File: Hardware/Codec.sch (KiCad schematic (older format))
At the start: 11 parts, among them U301 SGTL5000XNAA3

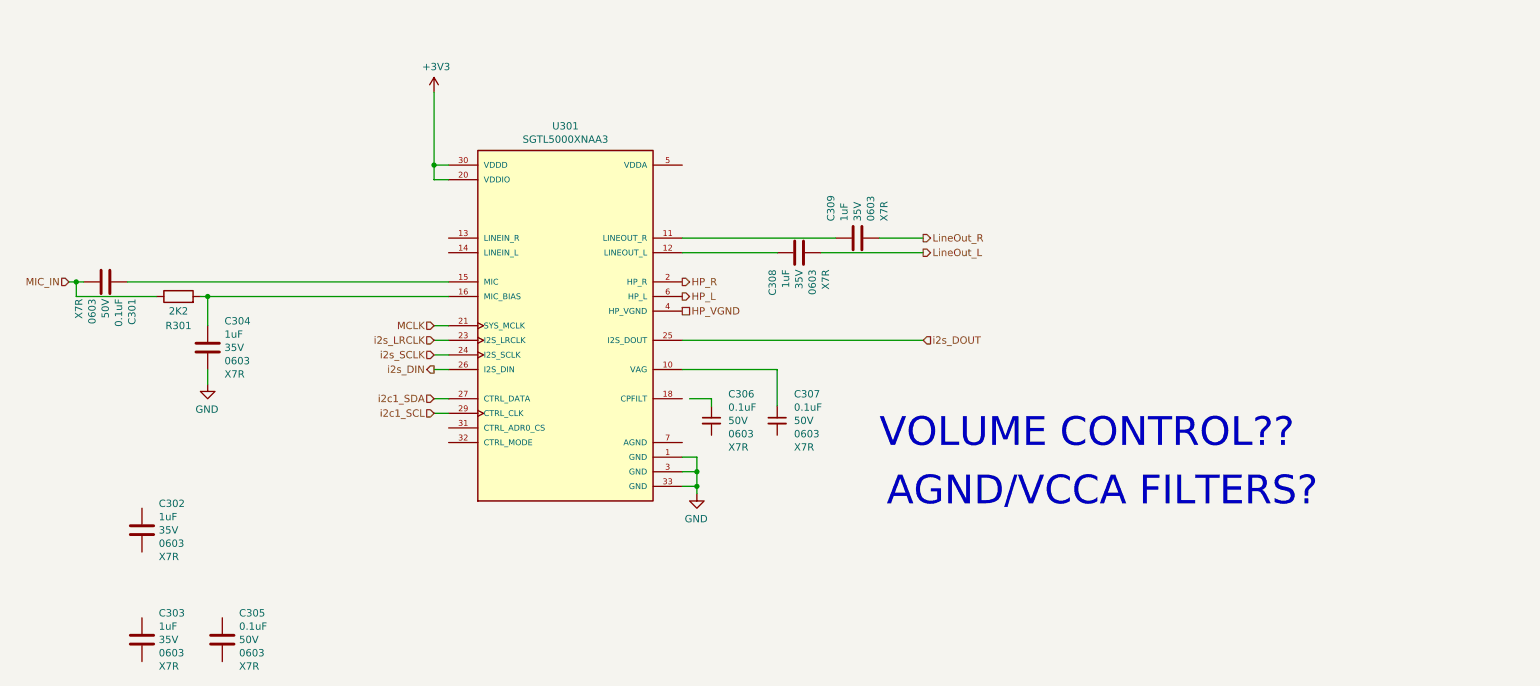
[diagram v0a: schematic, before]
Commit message: Commit berfore merge back with power fix.
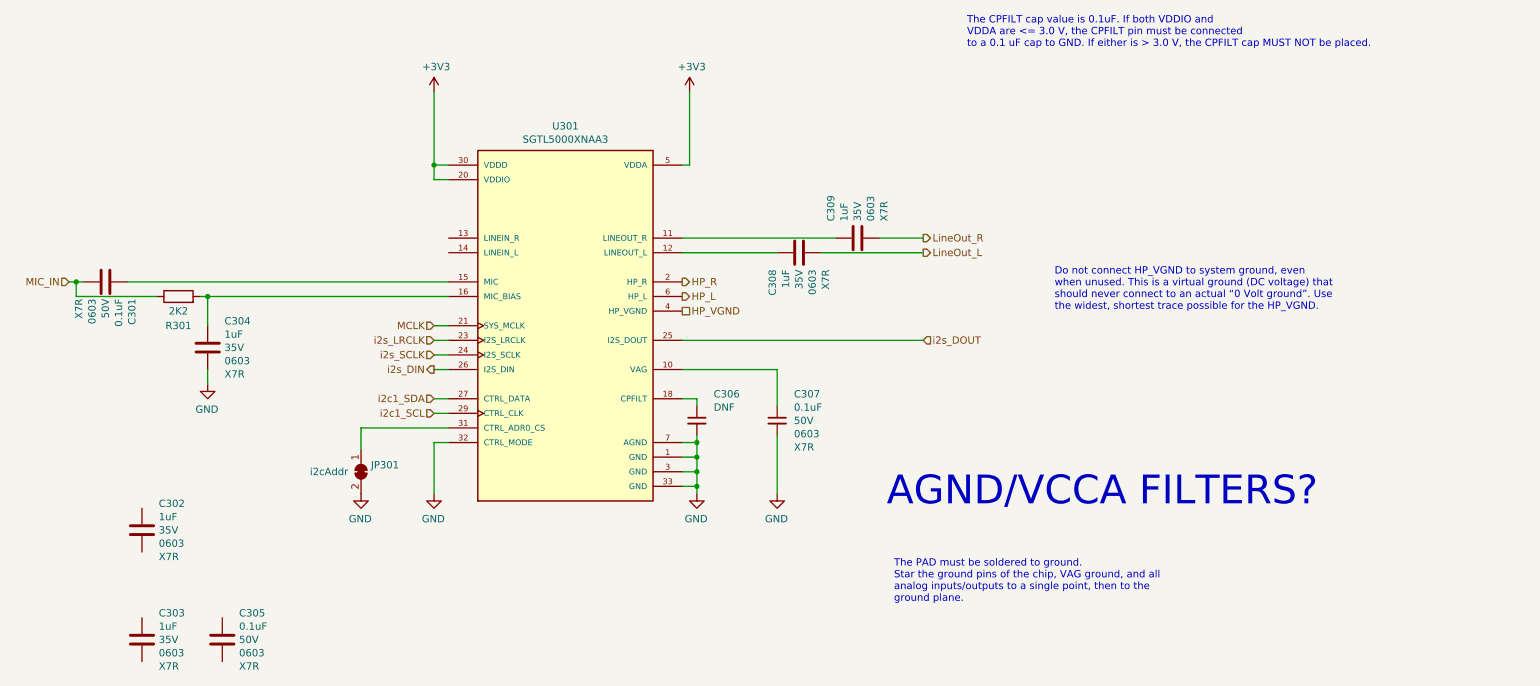
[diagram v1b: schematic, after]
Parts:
- added JP301: i2cAddr, Jumper:SolderJumper-2_P1.3mm_Bridged_RoundedPad1.0x1.5mm, symbol Jumper:SolderJumper_2_Bridged
- C306: value 0.1uF -> DNF; footprint Capacitor_SMD:C_0603_1608Metric -> Capacitor_SMD:C_0402_1005Metric; DPN 399-6856-1-ND -> (none); MPN C0603C104K5RACAUTO -> (none); Pkg 0603 -> (none); TCoff X7R -> (none); Tol 50V -> (none)
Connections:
- net +3V3: now also U301.5 (VDDA)
- net GND: now also C306.2, C307.2, U301.32 (CTRL_MODE), U301.7 (AGND), JP301.2 (B)
- net at U301.18 (CPFILT): now also C306.1
- net at U301.31 (CTRL_ADR0_CS): now also JP301.1 (A)
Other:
- note added: "Do not connect HP_VGND to system ground, even\nwhen unused. This is a virtual ground (DC voltage) that\nshould never connect to an actual “0 Volt ground”. Use\nthe widest, shortest trace possible for the HP_VGND.\n"
- note added: "The CPFILT cap value is 0.1uF. If both VDDIO and\nVDDA are <= 3.0 V, the CPFILT pin must be connected \nto a 0.1 uF cap to GND. If either is > 3.0 V, the CPFILT cap MUST NOT be placed."
- note added: "The PAD must be soldered to ground.\nStar the ground pins of the chip, VAG ground, and all\nanalog inputs/outputs to a single point, then to the\nground plane.\n"
- note removed: "VOLUME CONTROL??"
- moved on the sheet: C306
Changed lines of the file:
@@
 L Device:C_Small C?
 U 1 1 61383D31
-P 6250 4100
+P 6150 4100
 AR Path="/611E335F/61383D31" Ref="C?"  Part="1"
 AR Path="/611E3218/611E32E1/61383D31" Ref="C306"  Part="1"
-F 0 "C306" H 6365 4282 50  0000 L CNN
-F 1 "0.1uF" H 6365 4191 50  0000 L CNN
-F 2 "Capacitor_SMD:C_0603_1608Metric" H 6288 3950 50  0001 C CNN
-F 3 "~" H 6250 4100 50  0001 C CNN
-F 4 "C0603C104K5RACAUTO" H 6250 4100 50  0001 C CNN "MPN"
-F 5 "399-6856-1-ND" H 6250 4100 50  0001 C CNN "DPN"
-F 6 "50V" H 6365 4100 50  0000 L CNN "Tol"
-F 7 "0603" H 6365 4009 50  0000 L CNN "Pkg"
-F 8 "X7R" H 6365 3918 50  0000 L CNN "TCoff"
-	1    6250 4100
+F 0 "C306" H 6265 4282 50  0000 L CNN
+F 1 "DNF" H 6265 4191 50  0000 L CNN
+F 2 "Capacitor_SMD:C_0402_1005Metric" H 6188 3950 50  0001 C CNN
+F 3 "~" H 6150 4100 50  0001 C CNN
+F 4 "" H 6150 4100 50  0001 C CNN "MPN"
+F 5 "" H 6150 4100 50  0001 C CNN "DPN"
+F 6 "" H 6265 4100 50  0000 L CNN "Tol"
+F 7 "" H 6265 4009 50  0000 L CNN "Pkg"
+F 8 "" H 6265 3918 50  0000 L CNN "TCoff"
+	1    6150 4100
 	1    0    0    -1
 $EndComp
@@
 	6700 3750 6700 4000
 Wire Wire Line
-	6100 3950 6250 3950
-Wire Wire Line
-	6250 3950 6250 4000
+	6150 3950 6150 4000
 Text HLabel 1850 3150 0    50   Input ~ 0
 MIC_IN
@@
 	6150 4350 6150 4450
 Connection ~ 6150 4450
-Text Notes 7400 4300 0    197  ~ 0
-VOLUME CONTROL??
 Wire Wire Line
 	4450 2350 4350 2350
@@
 Text Notes 7450 4700 0    197  ~ 0
 AGND/VCCA FILTERS?
+Wire Wire Line
+	6050 4250 6150 4250
+Wire Wire Line
+	6150 4250 6150 4350
+Connection ~ 6150 4350
+$Comp
+L power:GND #PWR?
+U 1 1 616A5FE3
+P 4350 4600
+AR Path="/611E3335/616A5FE3" Ref="#PWR?"  Part="1"
+AR Path="/611E3218/611E32E1/616A5FE3" Ref="#PWR0179"  Part="1"
+F 0 "#PWR0179" H 4350 4350 50  0001 C CNN
+F 1 "GND" H 4355 4427 50  0000 C CNN
+F 2 "" H 4350 4600 50  0001 C CNN
+F 3 "" H 4350 4600 50  0001 C CNN
+	1    4350 4600
+	-1   0    0    -1
+$EndComp
+Wire Wire Line
+	4450 4250 4350 4250
+Wire Wire Line
+	4350 4250 4350 4600
+$Comp
+L Jumper:SolderJumper_2_Bridged JP301
+U 1 1 616A9E90
+P 3850 4450
+F 0 "JP301" V 3804 4518 50  0000 L CNN
+F 1 "i2cAddr" V 3850 4100 50  0000 L CNN
+F 2 "Jumper:SolderJumper-2_P1.3mm_Bridged_RoundedPad1.0x1.5mm" H 3850 4450 50  0001 C CNN
+F 3 "~" H 3850 4450 50  0001 C CNN
+	1    3850 4450
+	0    1    1    0
+$EndComp
+Wire Wire Line
+	3850 4150 3850 4300
+Wire Wire Line
+	3850 4150 4450 4150
+$Comp
+L power:GND #PWR?
+U 1 1 616AB03B
+P 3850 4600
+AR Path="/611E3335/616AB03B" Ref="#PWR?"  Part="1"
+AR Path="/611E3218/611E32E1/616AB03B" Ref="#PWR0180"  Part="1"
+F 0 "#PWR0180" H 3850 4350 50  0001 C CNN
+F 1 "GND" H 3855 4427 50  0000 C CNN
+F 2 "" H 3850 4600 50  0001 C CNN
+F 3 "" H 3850 4600 50  0001 C CNN
+	1    3850 4600
+	-1   0    0    -1
+$EndComp
+$Comp
+L power:+3V3 #PWR?
+U 1 1 616AD8A4
+P 6100 1850
+AR Path="/6123BB15/616AD8A4" Ref="#PWR?"  Part="1"
+AR Path="/611E335F/616AD8A4" Ref="#PWR?"  Part="1"
+AR Path="/611E3218/611E32E1/616AD8A4" Ref="#PWR0181"  Part="1"
+F 0 "#PWR0181" H 6100 1700 50  0001 C CNN
+F 1 "+3V3" H 6115 2023 50  0000 C CNN
+F 2 "" H 6100 1850 50  0001 C CNN
+F 3 "" H 6100 1850 50  0001 C CNN
+	1    6100 1850
+	1    0    0    -1
+$EndComp
+Wire Wire Line
+	6100 1850 6100 2350
+Wire Wire Line
+	6100 2350 6050 2350
+Wire Wire Line
+	6050 3950 6150 3950
+Text Notes 8000 1550 0    50   ~ 0
+The CPFILT cap value is 0.1uF. If both VDDIO and\nVDDA are <= 3.0 V, the CPFILT pin must be connected \nto a 0.1 uF cap to GND. If either is > 3.0 V, the CPFILT cap MUST NOT be placed.
+Wire Wire Line
+	6150 4200 6150 4250
+Connection ~ 6150 4250
+Text Notes 7500 5350 0    50   ~ 0
+The PAD must be soldered to ground.\nStar the ground pins of the chip, VAG ground, and all\nanalog inputs/outputs to a single point, then to the\nground plane.\n
+$Comp
+L power:GND #PWR?
+U 1 1 616B7426
+P 6700 4600
+AR Path="/611E3335/616B7426" Ref="#PWR?"  Part="1"
+AR Path="/611E3218/611E32E1/616B7426" Ref="#PWR0182"  Part="1"
+F 0 "#PWR0182" H 6700 4350 50  0001 C CNN
+F 1 "GND" H 6705 4427 50  0000 C CNN
+F 2 "" H 6700 4600 50  0001 C CNN
+F 3 "" H 6700 4600 50  0001 C CNN
+	1    6700 4600
+	-1   0    0    -1
+$EndComp
+Wire Wire Line
+	6700 4200 6700 4600
+Text Notes 8600 3350 0    50   ~ 0
+ Do not connect HP_VGND to system ground, even\nwhen unused. This is a virtual ground (DC voltage) that\nshould never connect to an actual “0 Volt ground”. Use\nthe widest, shortest trace possible for the HP_VGND.\n
 $EndSCHEMATC
